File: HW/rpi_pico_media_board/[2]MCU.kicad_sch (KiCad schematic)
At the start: 12 parts, among them J200 Conn_01x04_Pin, J201 Conn_01x03, SW200 SW_DPDT_XLX, U200 RaspberryPi_Pico, U202 mems-mic, U203 mems-mic

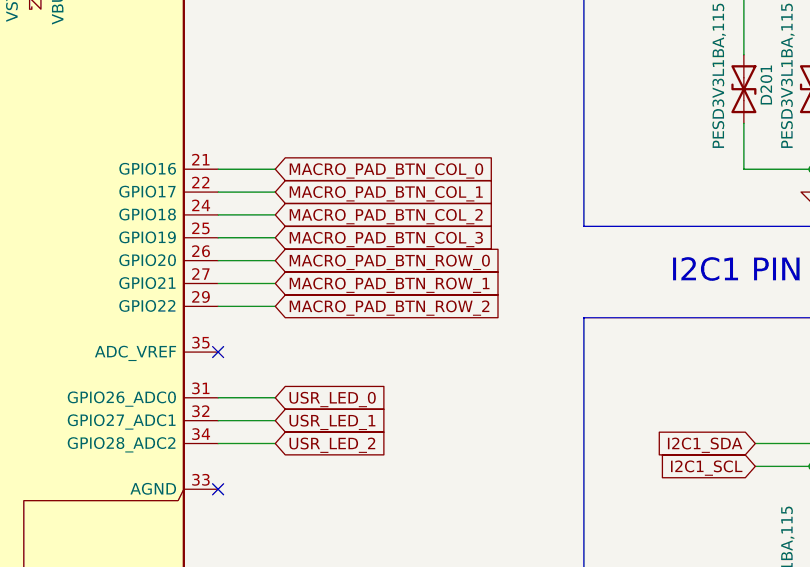
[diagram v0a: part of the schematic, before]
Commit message: Macro Pad routing
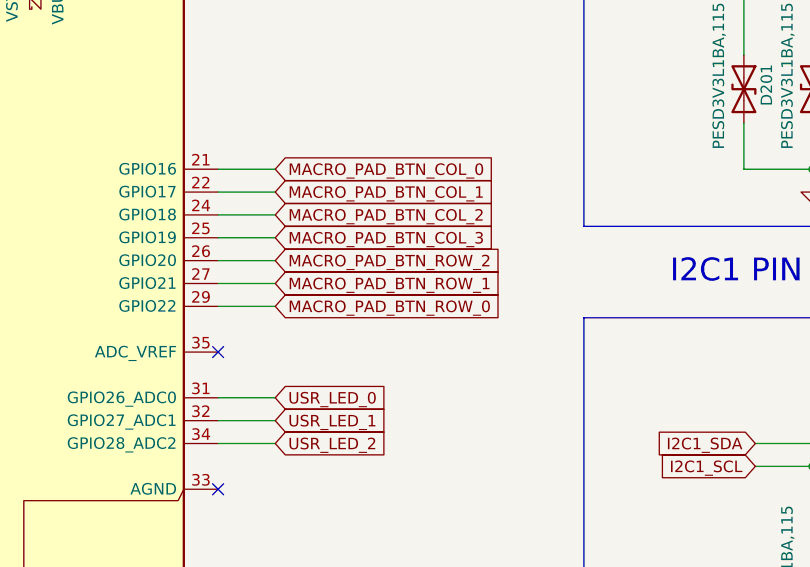
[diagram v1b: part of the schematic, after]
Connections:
- net MACRO_PAD_BTN_ROW_0: now also U200.29 (GPIO22); no longer U200.26 (GPIO20)
- net MACRO_PAD_BTN_ROW_2: now also U200.26 (GPIO20); no longer U200.29 (GPIO22)
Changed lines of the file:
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@@
+	(wire
+		(pts
+			(xy 176.53 92.71) (xy 182.88 92.71)
+		)
+		(stroke
+			(width 0)
+			(type default)
+		)
+	)
 	(wire
 		(pts
@@
 	(wire
 		(pts
+			(xy 176.53 90.17) (xy 182.88 90.17)
+		)
+		(stroke
+			(width 0)
+			(type default)
+		)
+	)
+	(wire
+		(pts
 			(xy 125.73 82.55) (xy 130.81 82.55)
 		)
@@
 	(wire
 		(pts
+			(xy 176.53 95.25) (xy 182.88 95.25)
+		)
+		(stroke
+			(width 0)
+			(type default)
+		)
+	)
+	(wire
+		(pts
 			(xy 250.19 135.89) (xy 242.57 135.89)
 		)
@@
 	(wire
 		(pts
-			(xy 176.53 90.17) (xy 182.88 90.17)
-		)
-		(stroke
-			(width 0)
-			(type default)
-		)
-	)
-	(wire
-		(pts
 			(xy 176.53 105.41) (xy 182.88 105.41)
 		)
@@
 	(wire
 		(pts
-			(xy 176.53 95.25) (xy 182.88 95.25)
-		)
-		(stroke
-			(width 0)
-			(type default)
-		)
-	)
-	(wire
-		(pts
 			(xy 26.67 140.97) (xy 26.67 154.94)
 		)
@@
 		(pts
 			(xy 176.53 107.95) (xy 182.88 107.95)
-		)
-		(stroke
-			(width 0)
-			(type default)
-		)
-	)
-	(wire
-		(pts
-			(xy 176.53 92.71) (xy 182.88 92.71)
 		)
 		(stroke
@@
 	(global_label "MACRO_PAD_BTN_ROW_0"
 		(shape input)
+		(at 182.88 95.25 0)
+		(fields_autoplaced yes)
+		(effects
+			(font
+				(size 1.27 1.27)
+			)
+			(justify left)
+		)
+		(property "Intersheetrefs" "${INTERSHEET_REFS}"
+			(at 208.6042 95.25 0)
+			(effects
+				(font
+					(size 1.27 1.27)
+				)
+				(justify left)
+				(hide yes)
+			)
+		)
+	)
+	(global_label "MACRO_PAD_BTN_ROW_2"
+		(shape input)
 		(at 182.88 90.17 0)
 		(fields_autoplaced yes)
@@
 			(effects
 				(font
-					(size 1.27 1.27)
-				)
-				(justify left)
-				(hide yes)
-			)
-		)
-	)
-	(global_label "MACRO_PAD_BTN_ROW_2"
-		(shape input)
-		(at 182.88 95.25 0)
-		(fields_autoplaced yes)
-		(effects
-			(font
-				(size 1.27 1.27)
-			)
-			(justify left)
-		)
-		(property "Intersheetrefs" "${INTERSHEET_REFS}"
-			(at 208.6042 95.25 0)
-			(effects
-				(font
